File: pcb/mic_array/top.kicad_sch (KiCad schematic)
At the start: 0 parts

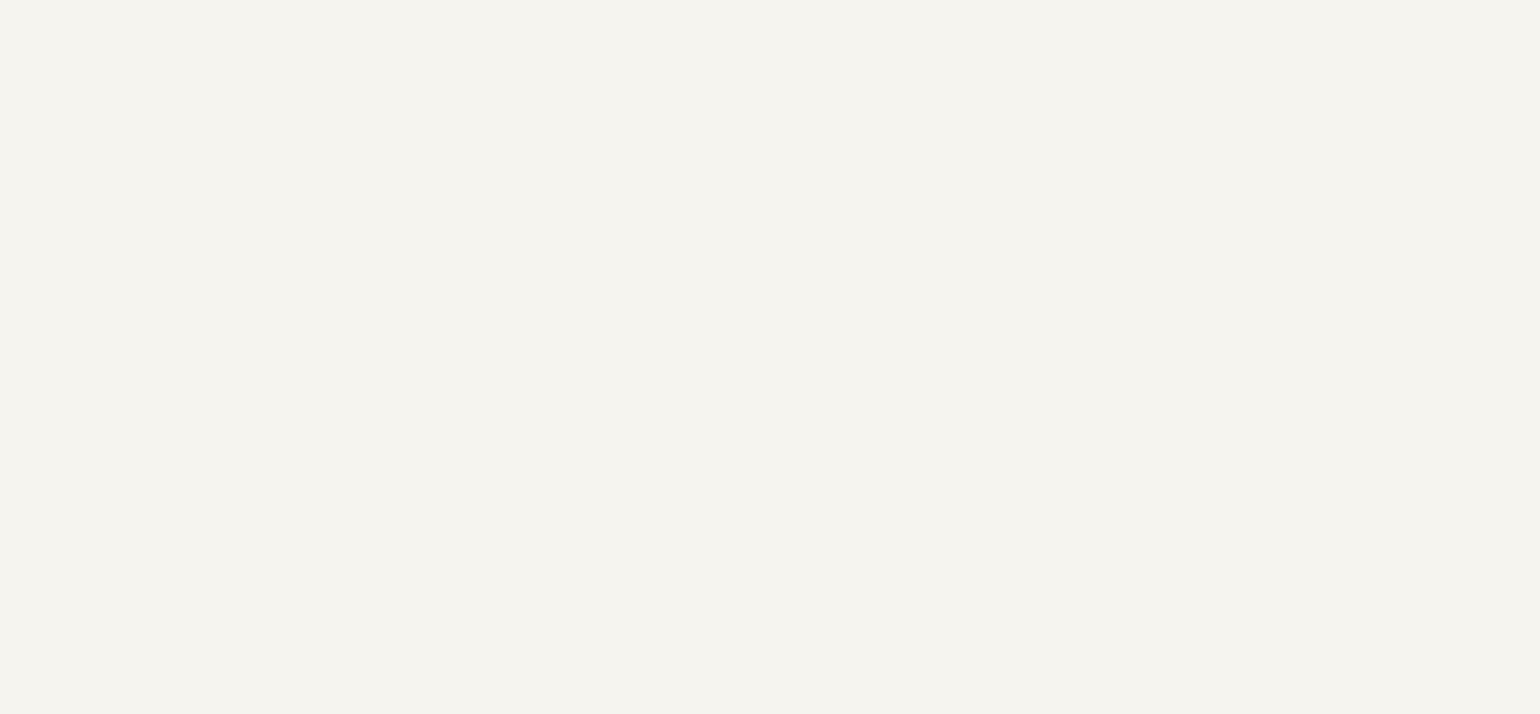
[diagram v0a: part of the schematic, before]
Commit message: Updated.
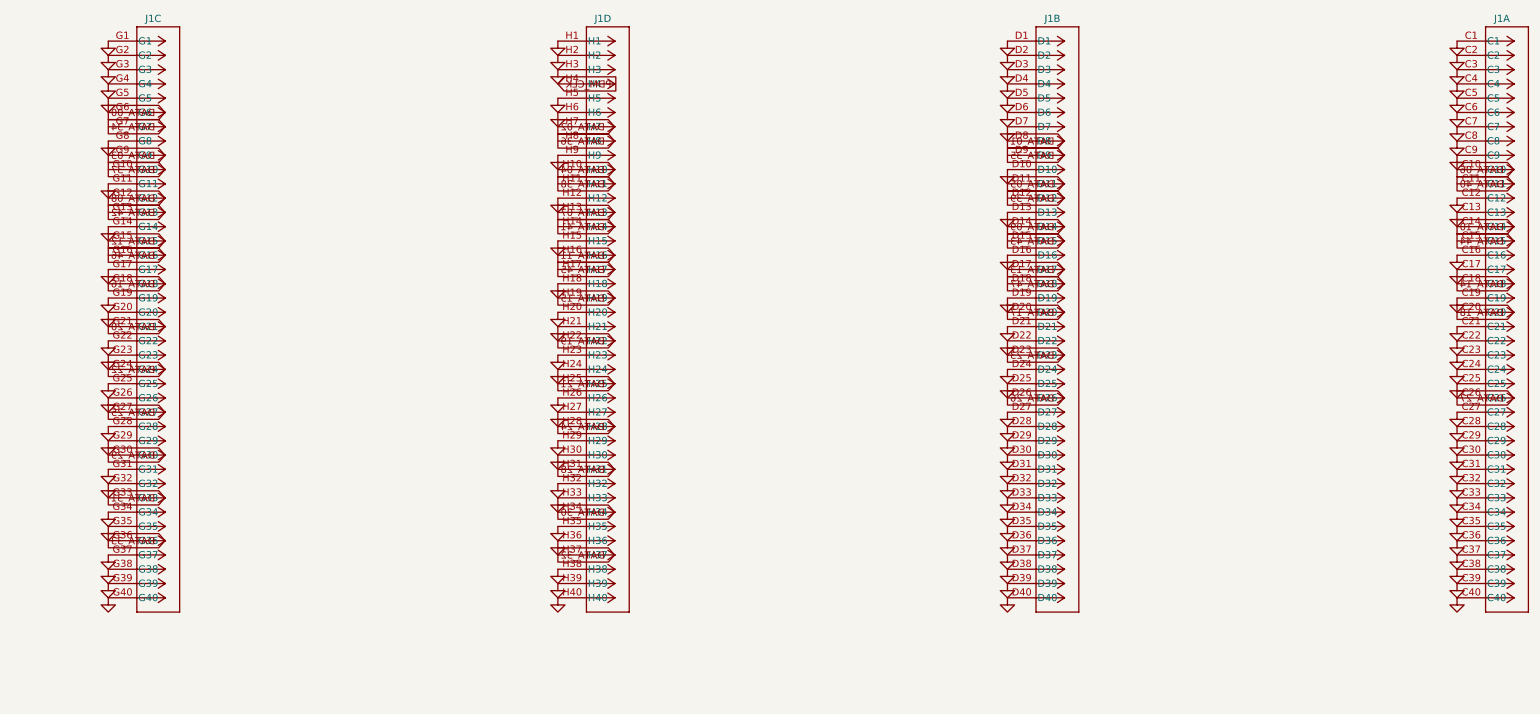
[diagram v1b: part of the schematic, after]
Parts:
- added J1: ASP-134604-01, Connector_Samtec:Samtec_FMC_ASP-134604-01_4x40_Vertical, symbol FMC_LPC:ASP-134604-01
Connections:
- new net DATA_00: J1.G6
- new net DATA_01: J1.D8
- new net DATA_02: J1.H7
- new net DATA_03: J1.G9
- new net DATA_04: J1.H10
- new net DATA_05: J1.D11
- new net DATA_06: J1.C10
- new net DATA_07: J1.H13
- new net DATA_08: J1.G12
- new net DATA_09: J1.D14
- new net DATA_10: J1.C14
- new net DATA_11: J1.H16
- new net DATA_12: J1.G15
- new net DATA_13: J1.D17
- new net DATA_14: J1.C18
- new net DATA_15: J1.H19
- new net DATA_16: J1.G18
- new net DATA_17: J1.D20
- new net DATA_18: J1.C20
- new net DATA_19: J1.H22
- new net DATA_20: J1.G21
- new net DATA_21: J1.H25
- new net DATA_22: J1.G24
- new net DATA_23: J1.D23
- new net DATA_24: J1.H28
- new net DATA_25: J1.G27
- new net DATA_26: J1.D26
- new net DATA_27: J1.C26
- new net DATA_28: J1.H31
- new net DATA_29: J1.G30
- new net DATA_30: J1.H34
- new net DATA_31: J1.G33
- new net DATA_32: J1.H37
- new net DATA_33: J1.G36
- new net DATA_34: J1.G7
- new net DATA_35: J1.D9
- new net DATA_36: J1.H8
- new net DATA_37: J1.G10
- new net DATA_38: J1.H11
- new net DATA_39: J1.D12
- new net DATA_40: J1.C11
- new net DATA_41: J1.H14
- new net DATA_42: J1.G13
- new net DATA_43: J1.D15
- new net DATA_44: J1.C15
- new net DATA_45: J1.H17
- new net DATA_46: J1.G16
- new net DATA_47: J1.D18
- new net GND: J1.C1, J1.C12, J1.C13, J1.C16, J1.C17, J1.C19, J1.C2, J1.C21, J1.C22, J1.C23, J1.C24, J1.C25, J1.C27, J1.C28, J1.C29, J1.C3, J1.C30, J1.C31, J1.C32, J1.C33, J1.C34, J1.C35, J1.C36, J1.C37, J1.C38, J1.C39, J1.C4, J1.C40, J1.C5, J1.C6, J1.C7, J1.C8, J1.C9, J1.D1, J1.D10, J1.D13, J1.D16, J1.D19, J1.D2, J1.D21, J1.D22, J1.D24, J1.D25, J1.D27, J1.D28, J1.D29, J1.D3, J1.D30, J1.D31, J1.D32, J1.D33, J1.D34, J1.D35, J1.D36, J1.D37, J1.D38, J1.D39, J1.D4, J1.D40, J1.D5, J1.D6, J1.D7, J1.G1, J1.G11, J1.G14, J1.G17, J1.G19, J1.G2, J1.G20, J1.G22, J1.G23, J1.G25, J1.G26, J1.G28, J1.G29, J1.G3, J1.G31, J1.G32, J1.G34, J1.G35, J1.G37, J1.G38, J1.G39, J1.G4, J1.G40, J1.G5, J1.G8, J1.H1, J1.H12, J1.H15, J1.H18, J1.H2, J1.H20, J1.H21, J1.H23, J1.H24, J1.H26, J1.H27, J1.H29, J1.H3, J1.H30, J1.H32, J1.H33, J1.H35, J1.H36, J1.H38, J1.H39, J1.H40, J1.H5, J1.H6, J1.H9
- new net PDM_CLK: J1.H4
